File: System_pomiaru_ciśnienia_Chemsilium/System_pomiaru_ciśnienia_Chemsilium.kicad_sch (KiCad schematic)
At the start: 7 parts, among them J1 PRESSURE_SENSOR_1, J3 PRESSURE_SENSOR_2, U1 ADS1115IDGS

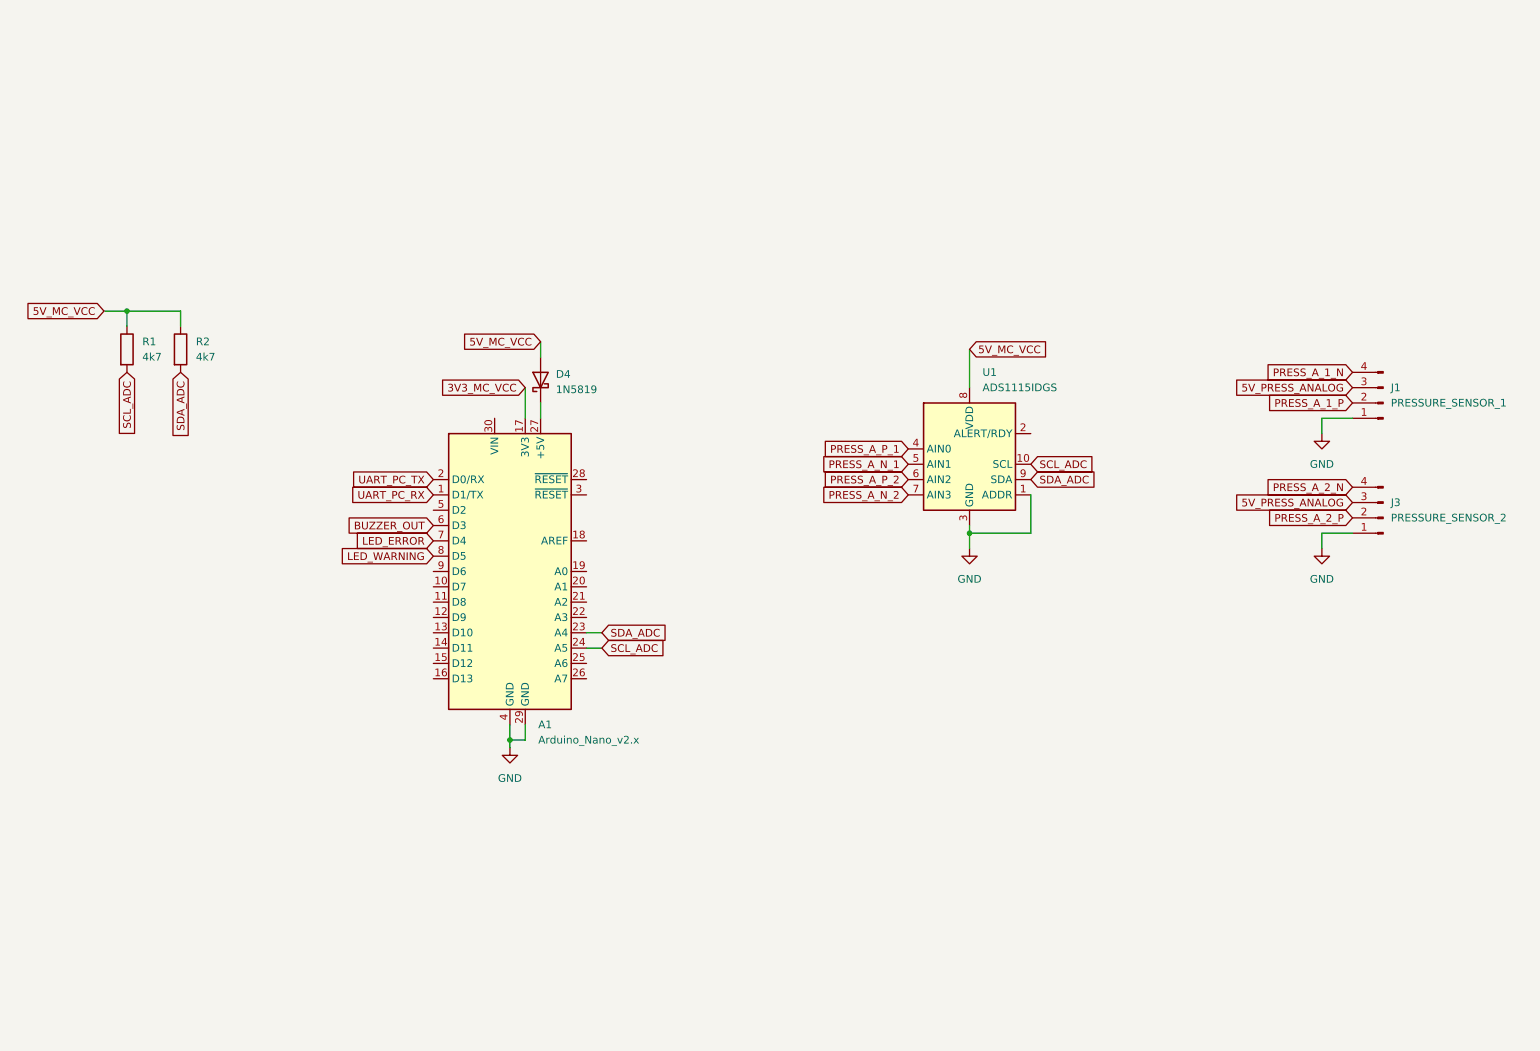
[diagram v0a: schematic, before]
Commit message: LPSN - backup backup
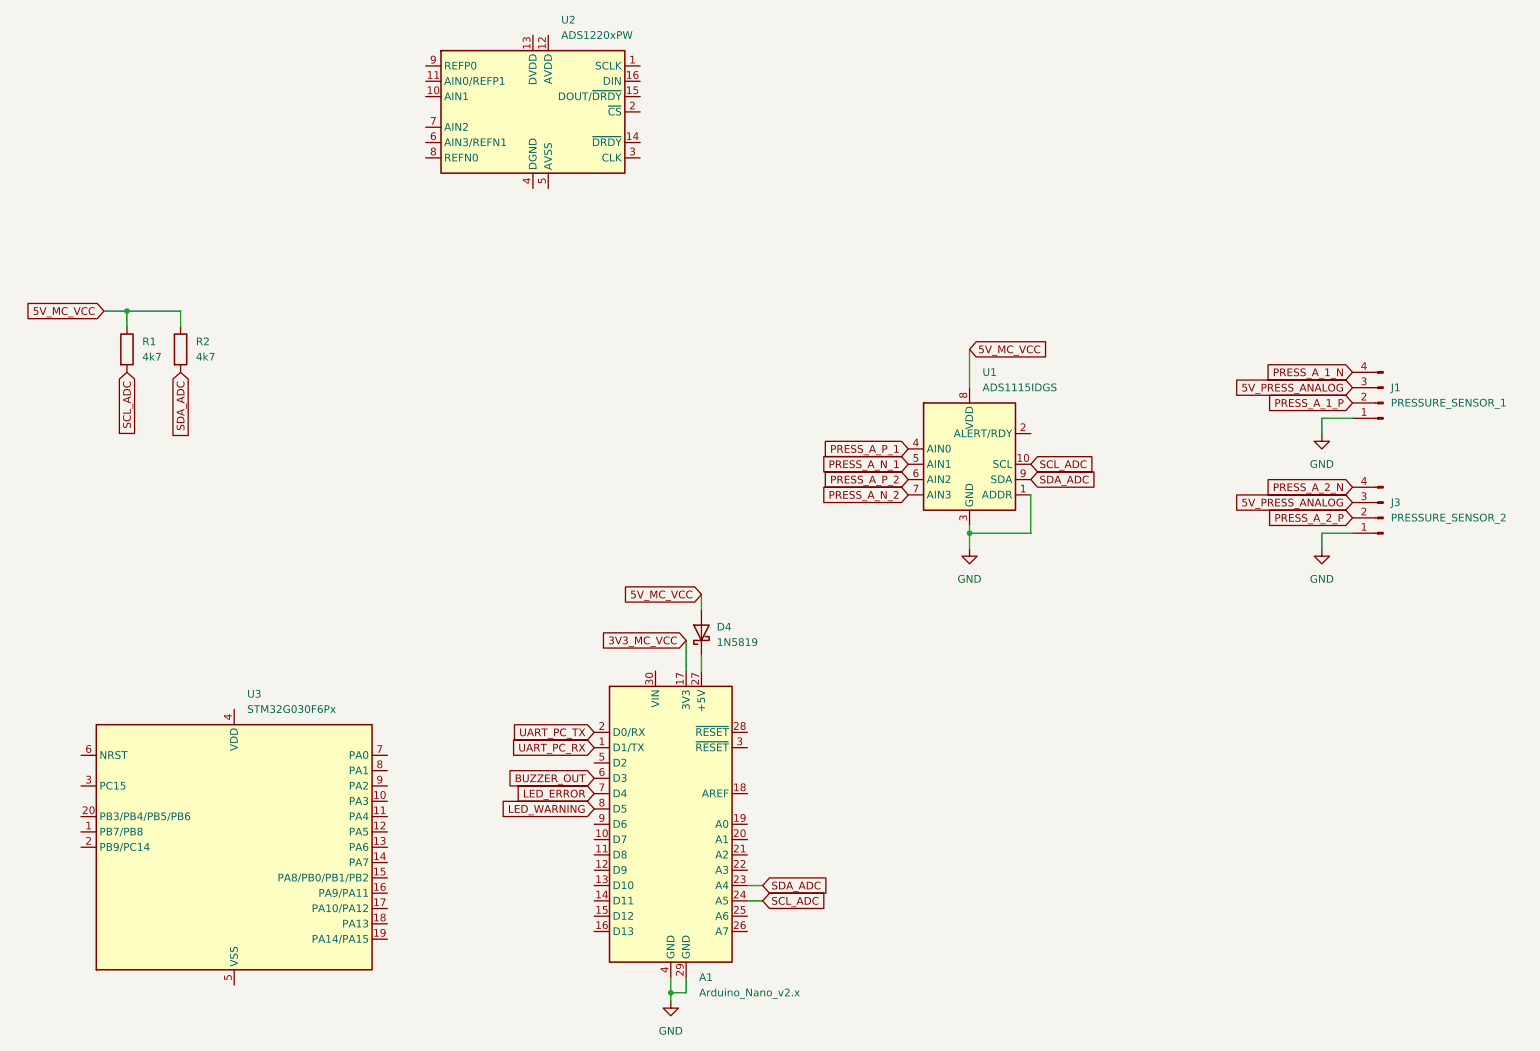
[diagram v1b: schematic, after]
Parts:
- added U2: ADS1220xPW, Package_SO:TSSOP-16_4.4x5mm_P0.65mm, symbol Analog_ADC:ADS1220xPW
- added U3: STM32G030F6Px, Package_SO:TSSOP-20_4.4x6.5mm_P0.65mm, symbol MCU_ST_STM32G0:STM32G030F6Px
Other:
- moved on the sheet: A1, D4
